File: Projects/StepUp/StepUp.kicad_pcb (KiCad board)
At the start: 2 copper layers, 47 parts, among them J1 Conn_01x02, J2 USB_B_Micro, U1 TMC2300-LA, U2 NCP1117-3.3_SOT223, U3 MIC2253, U4 W25Q128JVS, U5 RP2040, U6 COM-09032, Y1 ABM8-272-T3

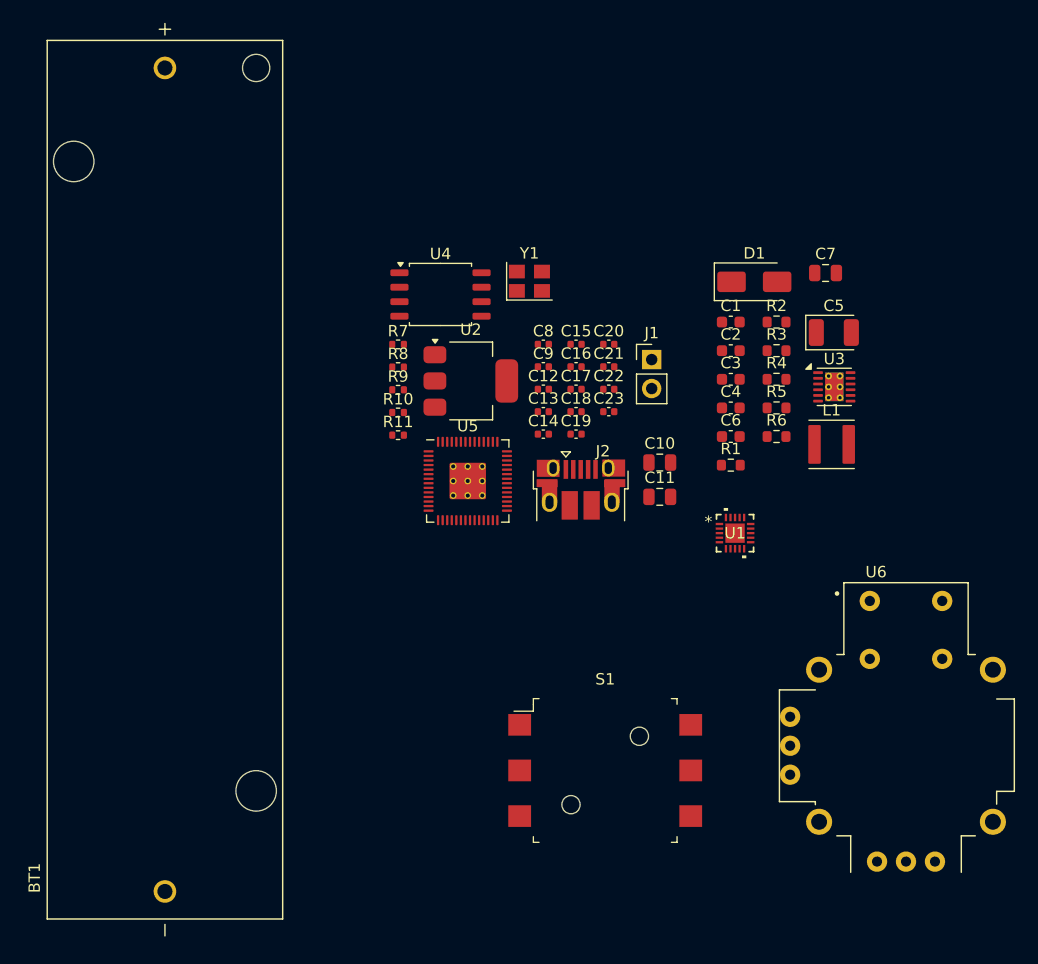
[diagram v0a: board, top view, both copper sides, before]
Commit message: feat(charge): Charge IC, USB ESD, sheet sections
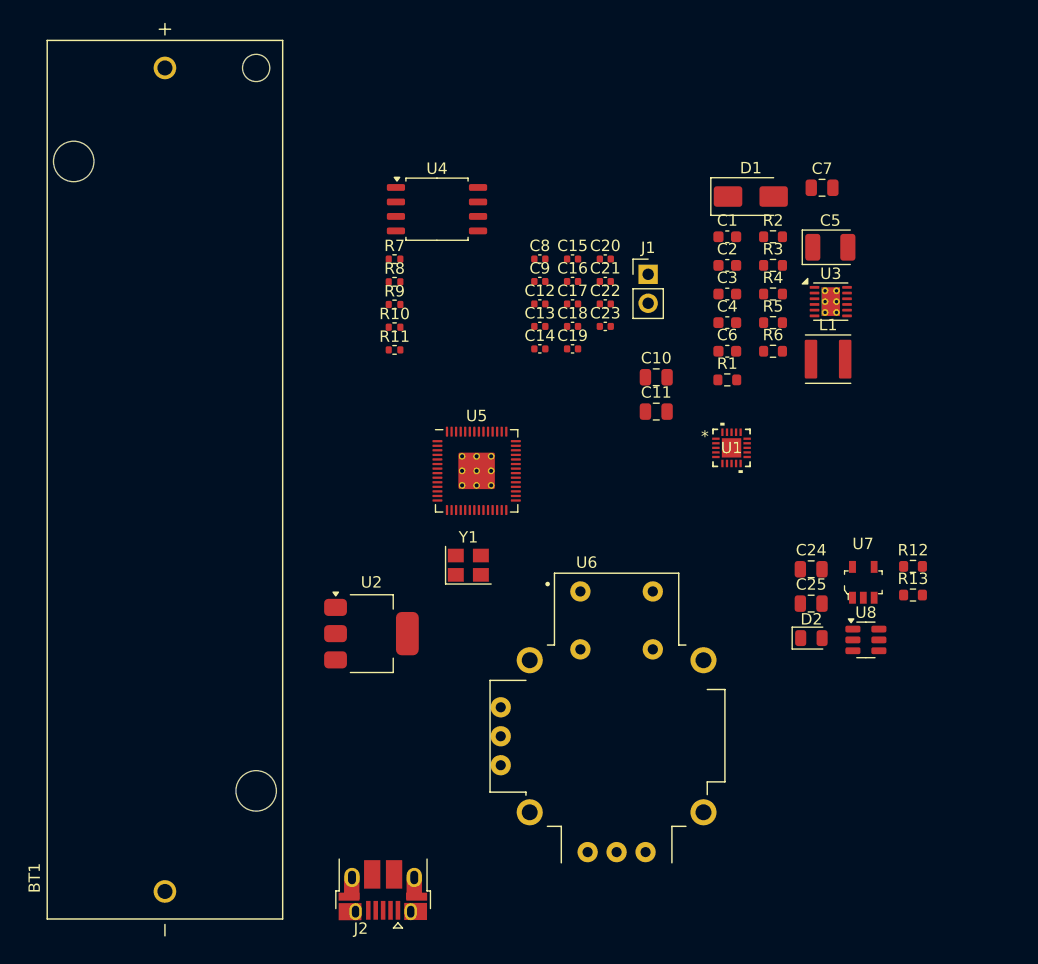
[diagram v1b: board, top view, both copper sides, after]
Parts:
- removed S1: JS5208, digikey-footprints:Switch_Nav_12.4x12.4mm_SMD_JS5208
- added C24: 4.7u, Capacitor_SMD:C_0805_2012Metric, F.Cu at (161.1, 112.9)
- added C25: 4.7u, Capacitor_SMD:C_0805_2012Metric, F.Cu at (161.1, 115.9)
- added D2: LED, LED_SMD:LED_0805_2012Metric, F.Cu at (161.1, 118.9)
- added R12: RProg, Resistor_SMD:R_0603_1608Metric, F.Cu at (170.0, 112.6)
- added R13: Rled, Resistor_SMD:R_0603_1608Metric, F.Cu at (170.0, 115.1)
- added U7: MCP73832T-2ACI_OT, digikey-footprints:SOT-753, F.Cu at (165.6, 114.0)
- added U8: USBLC6-2SC6, Package_TO_SOT_SMD:SOT-23-6, F.Cu at (165.9, 119.0)
- moved J2 39.2 mm to (123.5, 141.0), turned to 180 degrees
- moved Y1 25.5 mm to (131.0, 112.5)
- moved U6 25.4 mm to (144.0, 127.5)
- moved U2 23.8 mm to (122.5, 118.5)
- moved C10 7.48 mm to (147.5, 96.0)
- moved C15 7.48 mm to (140.1, 85.6)
- moved C20 7.48 mm to (143.0, 85.6)
- moved R10 7.48 mm to (124.5, 91.6)
- moved R3 7.48 mm to (157.7, 86.2)
- moved R6 7.48 mm to (157.7, 93.7)
- moved R7 7.48 mm to (124.5, 85.7)
- moved R8 7.48 mm to (124.5, 87.6)
- moved U3 7.48 mm to (162.8, 89.4)
- moved C2 7.48 mm to (153.7, 86.2)
- moved C6 7.48 mm to (153.7, 93.7)
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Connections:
- BT1 pad N: unconnected-(BT1-PadN) -> GND
- BT1 pad P: unconnected-(BT1-PadP) -> /Power/Vbat
- J2 pad 2: /Power/USB_D- -> /Power/USB_D-_IN
- J2 pad 3: /Power/USB_D+ -> /Power/USB_D+_IN
